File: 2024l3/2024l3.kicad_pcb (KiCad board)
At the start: 2 copper layers, 133 x 90.5 mm, 40 parts, among them J1 Conn_01x06, J2 TOF 0, J3 TOF 1, J4 TOF 2, J5 TOF 3, SW1 SW_SPDT, SW2 SW_SPDT, SW3 SW_SPDT, SW4 SW_SPDT, SW5 SW_SPDT, SW6 SW_SPDT, U1 OpenMV, U2 4754, U3 xiao-esp32c3, U4 Adafruit Featherwing, U5 Teensy 4.0, U6 xiao-esp32c3

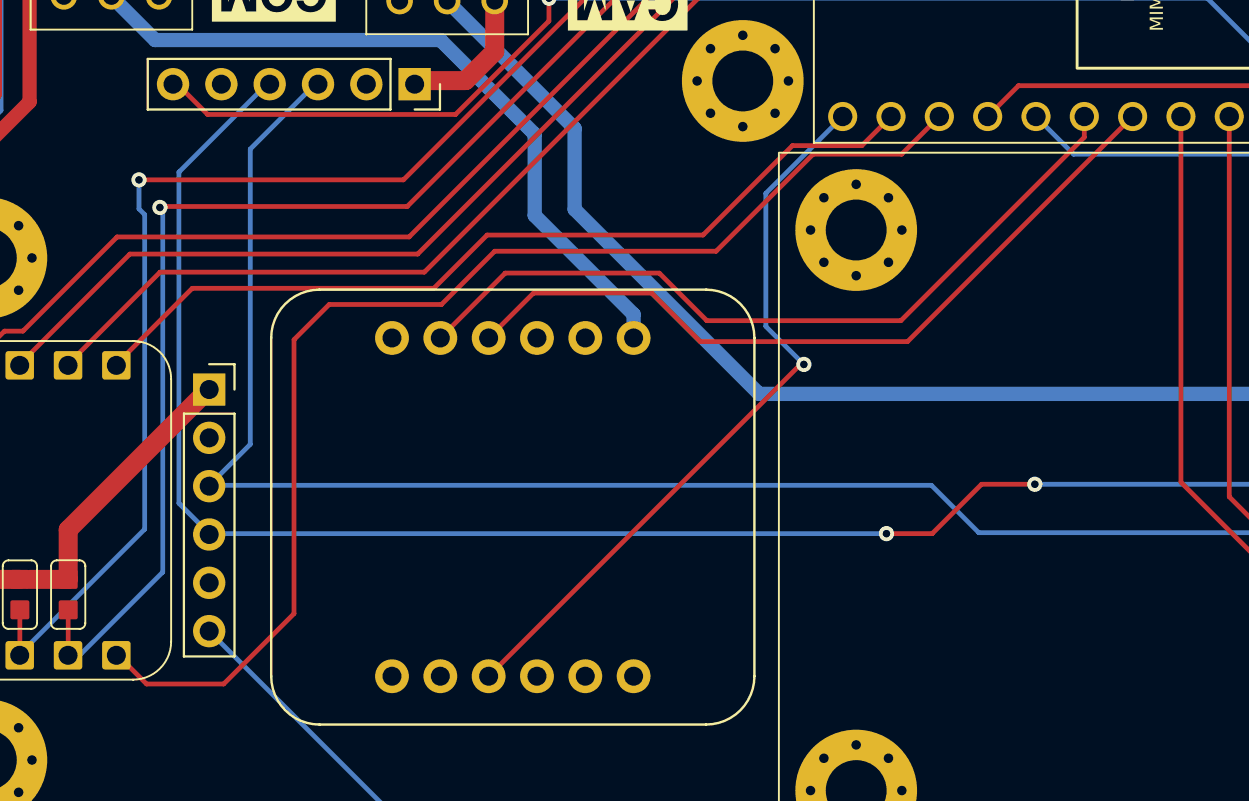
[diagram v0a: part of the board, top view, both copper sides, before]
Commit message: L1 Revert
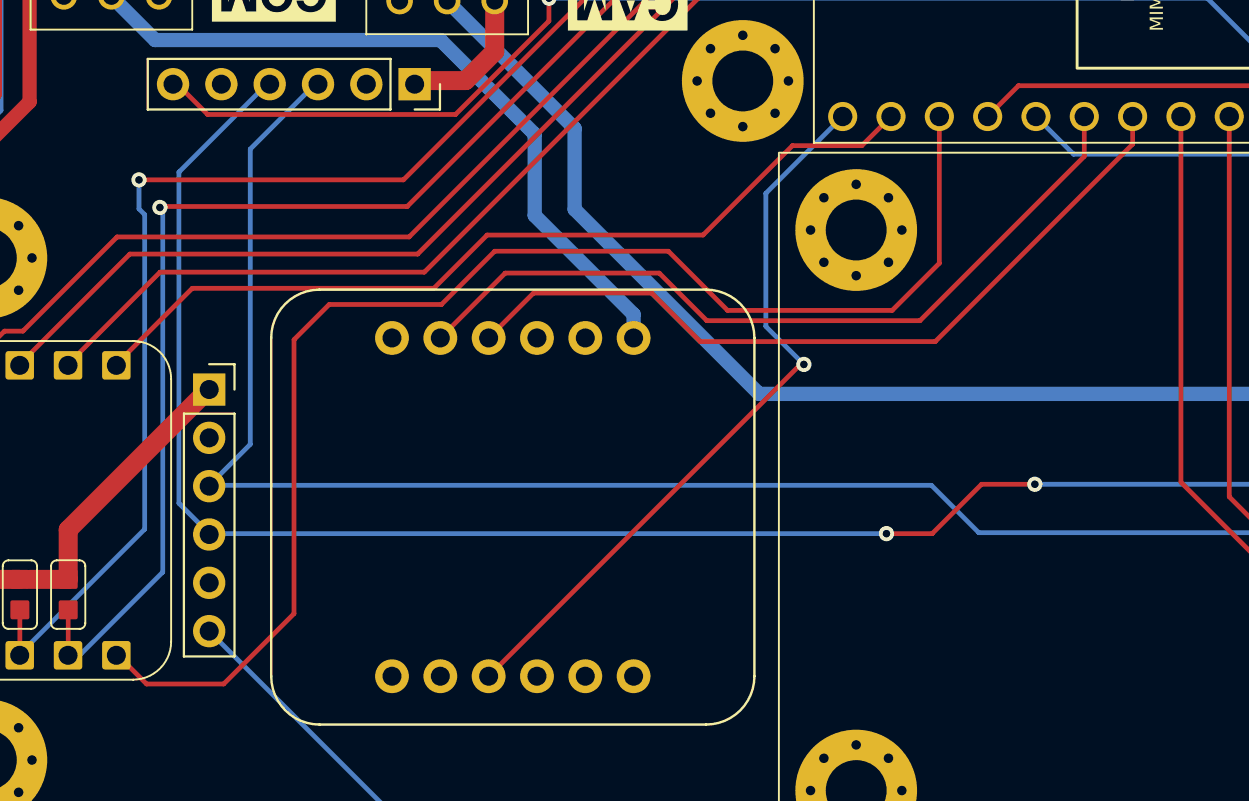
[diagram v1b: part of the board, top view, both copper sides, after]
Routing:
- net /ESP2 TX: track 64.7 -> 71.8 mm
- net /COM SCL: track 40.8 -> 41.6 mm
- net /COM SDA: track 41.4 -> 42.0 mm
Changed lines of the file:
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@@
   (segment (start 165.735 84.108) (end 165.735 88.244) (width 0.25) (layer "F.Cu") (net 45))
   (segment (start 165.735 88.244) (end 165.683 88.296) (width 0.25) (layer "F.Cu") (net 45))
-  (segment (start 158.115 84.108) (end 146.285 95.938) (width 0.25) (layer "F.Cu") (net 47))
+  (segment (start 132.835 93.388) (end 126.625 93.388) (width 0.25) (layer "F.Cu") (net 47))
+  (segment (start 147.738 95.938) (end 135.385 95.938) (width 0.25) (layer "F.Cu") (net 47))
+  (segment (start 126.625 93.388) (end 124.265 95.748) (width 0.25) (layer "F.Cu") (net 47))
+  (segment (start 158.115 85.561) (end 147.738 95.938) (width 0.25) (layer "F.Cu") (net 47))
   (segment (start 135.385 95.938) (end 132.835 93.388) (width 0.25) (layer "F.Cu") (net 47))
-  (segment (start 132.835 93.388) (end 126.625 93.388) (width 0.25) (layer "F.Cu") (net 47))
-  (segment (start 126.625 93.388) (end 124.265 95.748) (width 0.25) (layer "F.Cu") (net 47))
-  (segment (start 146.285 95.938) (end 135.385 95.938) (width 0.25) (layer "F.Cu") (net 47))
-  (segment (start 155.575 85.198) (end 155.575 84.108) (width 0.25) (layer "F.Cu") (net 48))
-  (segment (start 135.735 94.838) (end 145.935 94.838) (width 0.25) (layer "F.Cu") (net 48))
-  (segment (start 145.935 94.838) (end 155.575 85.198) (width 0.25) (layer "F.Cu") (net 48))
+  (segment (start 158.115 84.108) (end 158.115 85.561) (width 0.25) (layer "F.Cu") (net 47))
   (segment (start 133.235 92.338) (end 135.735 94.838) (width 0.25) (layer "F.Cu") (net 48))
+  (segment (start 146.938 94.838) (end 155.575 86.201) (width 0.25) (layer "F.Cu") (net 48))
+  (segment (start 135.735 94.838) (end 146.938 94.838) (width 0.25) (layer "F.Cu") (net 48))
+  (segment (start 121.725 95.748) (end 125.135 92.338) (width 0.25) (layer "F.Cu") (net 48))
   (segment (start 125.135 92.338) (end 133.235 92.338) (width 0.25) (layer "F.Cu") (net 48))
-  (segment (start 121.725 95.748) (end 125.135 92.338) (width 0.25) (layer "F.Cu") (net 48))
+  (segment (start 155.575 86.201) (end 155.575 84.108) (width 0.25) (layer "F.Cu") (net 48))
   (segment (start 140.835 97.138) (end 140.655 97.138) (width 0.25) (layer "F.Cu") (net 53))
   (segment (start 140.655 97.138) (end 124.265 113.528) (width 0.25) (layer "F.Cu") (net 53))
@@
   (segment (start 121.385 93.138) (end 124.185 90.338) (width 0.25) (layer "F.Cu") (net 91))
   (segment (start 135.535 90.338) (end 140.235 85.638) (width 0.25) (layer "F.Cu") (net 91))
-  (segment (start 147.955 84.108) (end 145.975 86.088) (width 0.25) (layer "F.Cu") (net 92))
-  (segment (start 114.035 110.238) (end 110.335 113.938) (width 0.25) (layer "F.Cu") (net 92))
-  (segment (start 121.785 93.988) (end 115.885 93.988) (width 0.25) (layer "F.Cu") (net 92))
-  (segment (start 110.335 113.938) (end 106.285 113.938) (width 0.25) (layer "F.Cu") (net 92))
-  (segment (start 136.221396 91.188) (end 124.585 91.188) (width 0.25) (layer "F.Cu") (net 92))
-  (segment (start 124.585 91.188) (end 121.785 93.988) (width 0.25) (layer "F.Cu") (net 92))
-  (segment (start 115.885 93.988) (end 114.035 95.838) (width 0.25) (layer "F.Cu") (net 92))
-  (segment (start 141.321396 86.088) (end 136.221396 91.188) (width 0.25) (layer "F.Cu") (net 92))
-  (segment (start 114.035 95.838) (end 114.035 110.238) (width 0.25) (layer "F.Cu") (net 92))
-  (segment (start 145.975 86.088) (end 141.321396 86.088) (width 0.25) (layer "F.Cu") (net 92))
-  (segment (start 106.285 113.938) (end 104.705 112.358) (width 0.25) (layer "F.Cu") (net 92))
+  (segment (start 124.585 91.188) (end 133.714 91.188) (width 0.25) (layer "F.Cu") (net 92))
+  (segment (start 110.335 113.938) (end 114.035 110.238) (width 0.25) (layer "F.Cu") (net 92))
+  (segment (start 121.785 93.988) (end 124.585 91.188) (width 0.25) (layer "F.Cu") (net 92))
+  (segment (start 114.035 110.238) (end 114.035 95.838) (width 0.25) (layer "F.Cu") (net 92))
+  (segment (start 114.035 95.838) (end 115.885 93.988) (width 0.25) (layer "F.Cu") (net 92))
+  (segment (start 147.955 91.821) (end 147.955 84.108) (width 0.25) (layer "F.Cu") (net 92))
+  (segment (start 106.285 113.938) (end 110.335 113.938) (width 0.25) (layer "F.Cu") (net 92))
+  (segment (start 136.826 94.3) (end 145.476 94.3) (width 0.25) (layer "F.Cu") (net 92))
+  (segment (start 115.885 93.988) (end 121.785 93.988) (width 0.25) (layer "F.Cu") (net 92))
+  (segment (start 104.705 112.358) (end 106.285 113.938) (width 0.25) (layer "F.Cu") (net 92))
+  (segment (start 145.476 94.3) (end 147.955 91.821) (width 0.25) (layer "F.Cu") (net 92))
+  (segment (start 133.714 91.188) (end 136.826 94.3) (width 0.25) (layer "F.Cu") (net 92))
   (zone locked (net 1) (net_name "GND") (layers "F&B.Cu") (hatch edge 0.5)
     (connect_pads yes (clearance 0.2))
